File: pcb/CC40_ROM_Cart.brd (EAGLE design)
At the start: 43.2 x 48 mm, 15 parts, among them IC1 SST39SF040APH/27CXX(X), X1 EXPANSION_PORT_CC40_EDGE

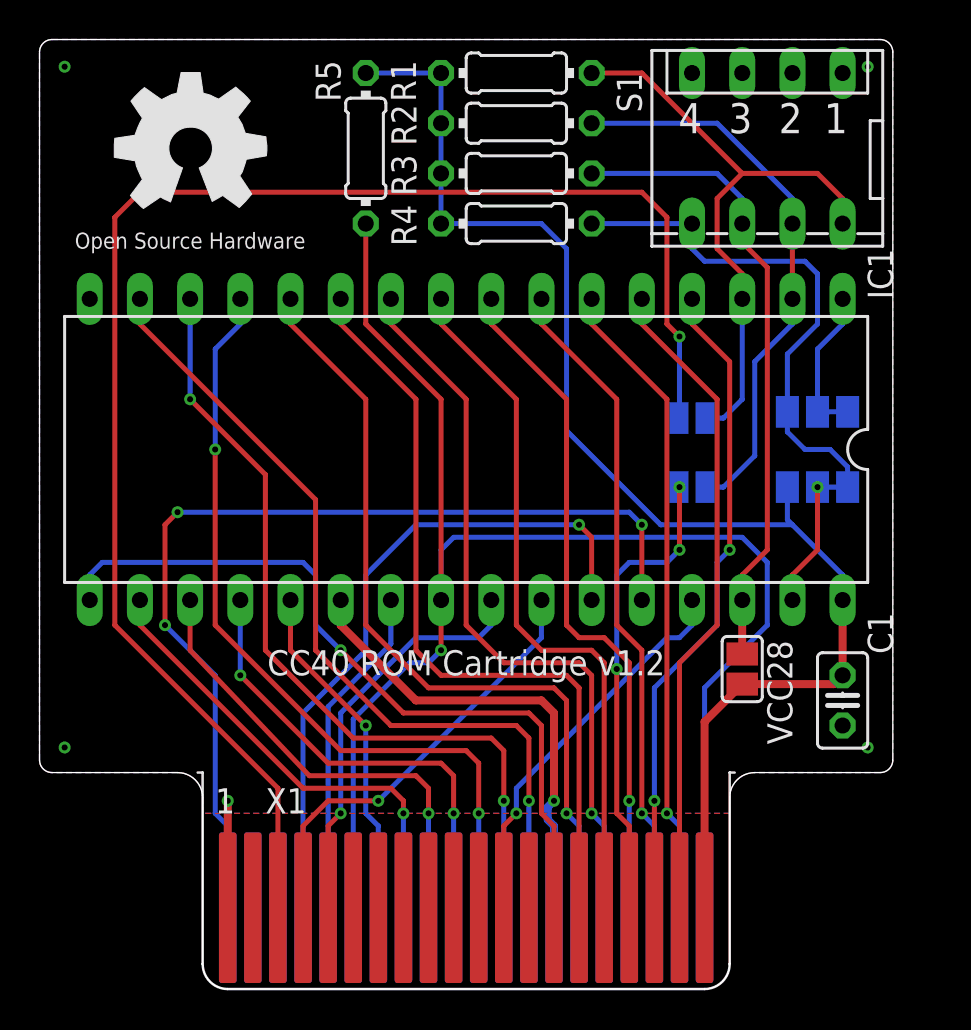
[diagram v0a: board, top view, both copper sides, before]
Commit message: Updated layouts and measurements
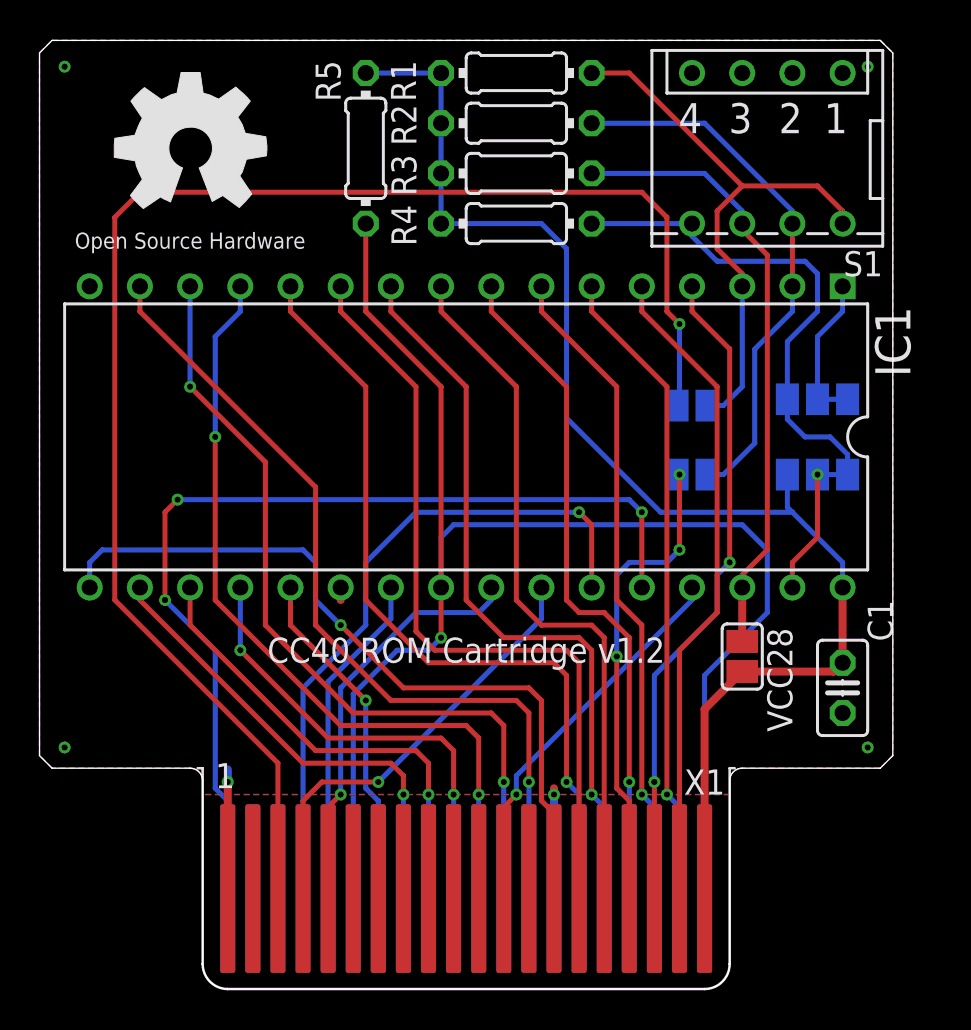
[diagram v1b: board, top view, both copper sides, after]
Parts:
- added P1: CC40_CARTN, ti-cc40-74-95:CC40_CART_NOHOLE
- IC1: value SST39SF040APH/27CXX(X) -> SST39SF040/27CXX(X); device memory-sst:DIL32 -> memory-sst:DIL32-RP
- S1: device switch-dil:DP-04 -> switch-dil-rp:DP-04
- X1: value EXPANSION_PORT_CC40_EDGE -> EXPANSION_PORT_CC40; device ti-cc40:MA20-2(.050) -> ti-cc40-74-95:MA20-2(.050)
- moved X1 1.27 mm to (0.00, 5.08)
- moved IC1 0.64 mm to (0.00, 27.9)
- moved P25.2 0.64 mm to (11.4, 29.5)
- moved P25.3 0.64 mm to (11.4, 26.0)
- moved SJ1 0.64 mm to (17.8, 26.0)
- moved VCC28 0.64 mm to (14.0, 16.8)
- moved C1 0.63 mm to (19.1, 15.2)
- moved SJ2 0.63 mm to (17.8, 29.8)
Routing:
- net GND: track 29.4 -> 13.7 mm
- net SA15: track 31.3 -> 29.6 mm
- net SA15': track 77.8 -> 76.2 mm
- net SA17: track 32.2 -> 31.2 mm
- net SA18': track 26.7 -> 25.7 mm
- net SA16: track 28.6 -> 27.6 mm
- net VBATT: track 0.00 -> 0.97 mm
- net VCC: track 69.0 -> 68.0 mm
- net A14: track 19.9 -> 19.2 mm
- net !CS: track 77.2 -> 76.6 mm
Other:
- outline, holes or cut-outs redrawn
